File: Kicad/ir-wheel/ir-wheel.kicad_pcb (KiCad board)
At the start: 2 copper layers, 58 x 25 mm, 20 parts, among them IC1 TTE-OPB606, IC2 TTE-OPB606, K1 RIGHT, K2 LEFT, P1 BOURNS-TC33X-200K, U1 MICROCHIP-MCP6541-SOT-23

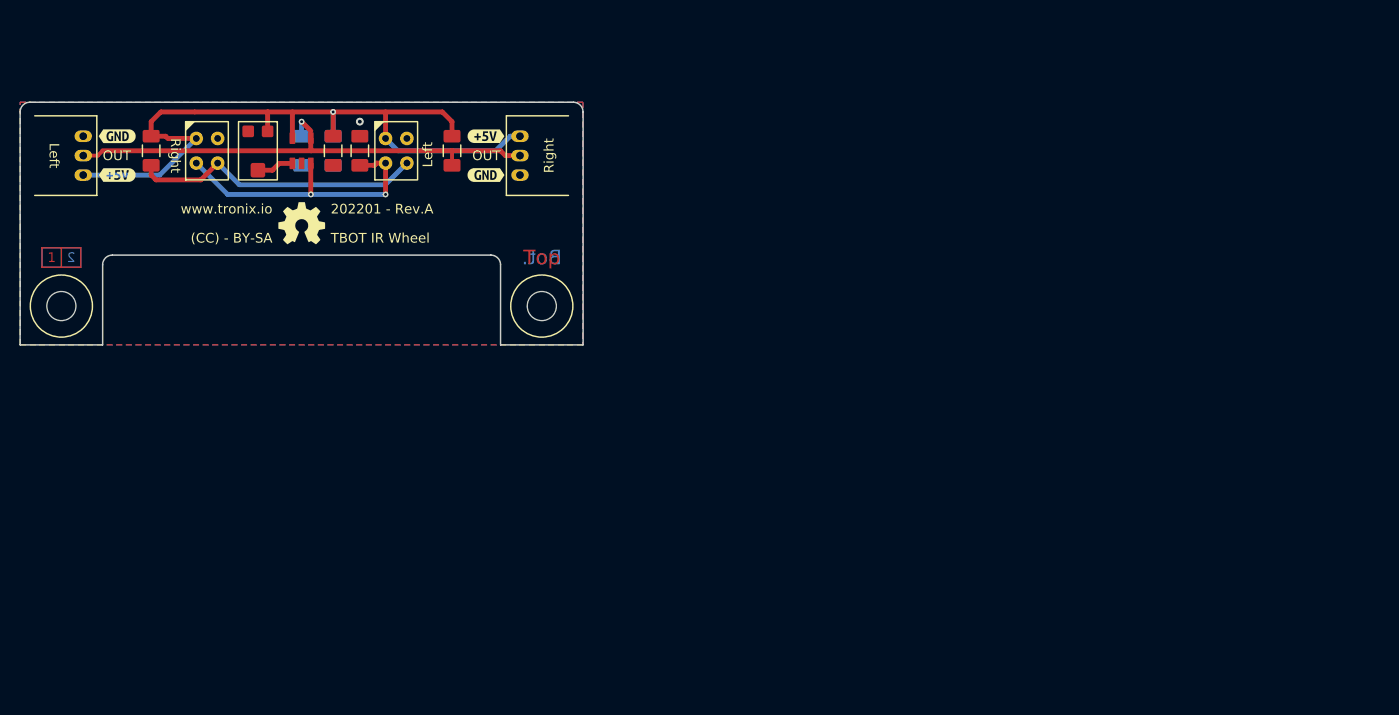
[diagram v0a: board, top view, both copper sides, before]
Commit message: Up
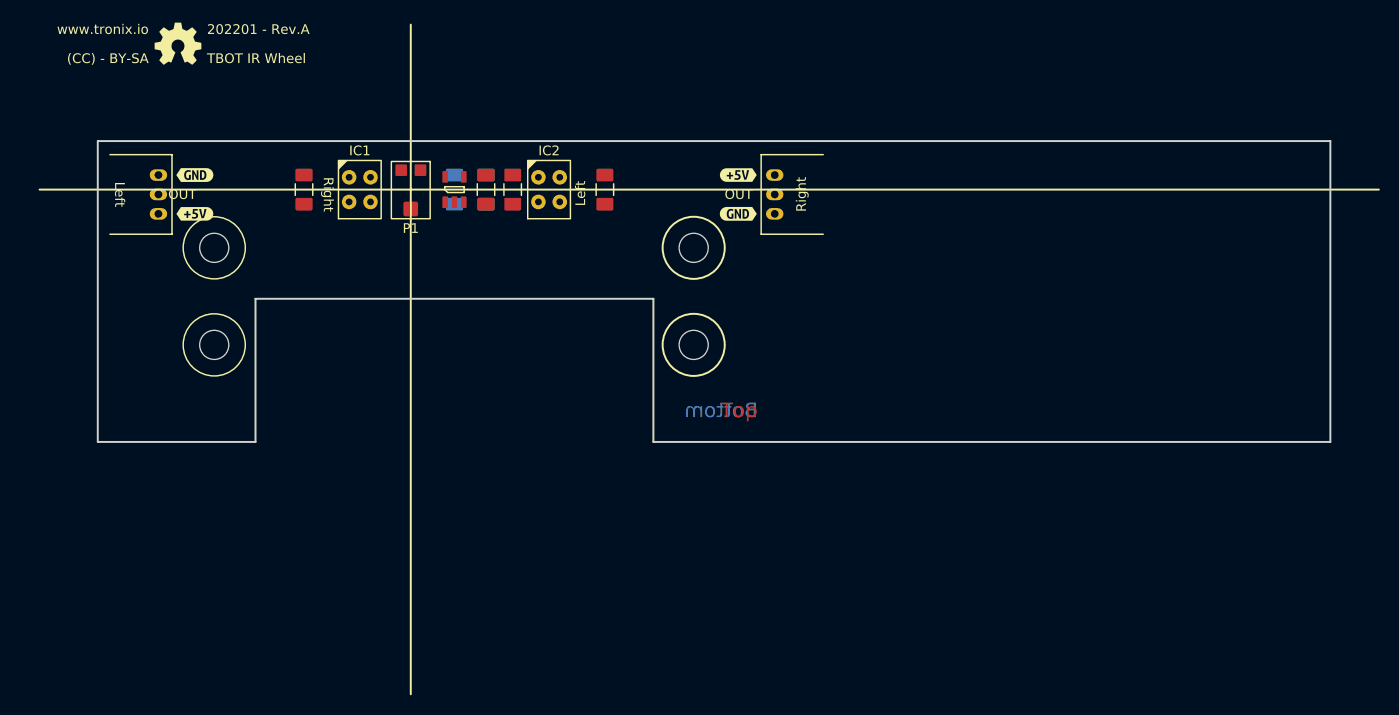
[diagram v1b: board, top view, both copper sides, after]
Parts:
- added H3: MOUNTING-HOLE-3MM-MASK, tronixio:MOUNTING-HOLE-3MM-MASK, F.Cu at (169.4, 100.0)
- added H4: MOUNTING-HOLE-3MM-MASK, tronixio:MOUNTING-HOLE-3MM-MASK, F.Cu at (169.4, 90.0)
- C1, C2, C3: footprint tronixio:CAPACITOR-1206 -> tronixio:CAPACITOR-SMD-1206
- H1, H2: value MOUNTING-HOLE-MASK-3MM -> MOUNTING-HOLE-3MM-MASK; footprint tronixio:M3-MASK -> tronixio:MOUNTING-HOLE-3MM-MASK
- IC1, IC2: value TTE-OPB606 -> OPB606; footprint tronixio:zzOPB-606 -> tronixio:OPB-606
- K1: value RIGHT -> Right
- K2: value LEFT -> Left
- P1: value BOURNS-TC33X-200K -> 200k; footprint tronixio:zzzTC33X -> tronixio:TC33X
- R1: footprint tronixio:RESISTOR-1206 -> tronixio:RESISTOR-SMD-1206
- R2: value 100K -> 100k; footprint tronixio:RESISTOR-1206 -> tronixio:RESISTOR-SMD-1206
- R3: value 10K -> 10k; footprint tronixio:RESISTOR-1206 -> tronixio:RESISTOR-SMD-1206
- U1: value MICROCHIP-MCP6541-SOT-23 -> MCP6541
- moved H2 34.0 mm to (120.0, 100.0)
- moved K2 26.6 mm to (177.8, 82.5)
- moved kibuzzard-629B8965 26.3 mm to (174.0, 82.5)
- moved kibuzzard-629B896F 26.3 mm to (174.0, 86.5)
- moved GB 22.5 mm to (116.2, 69.0)
- moved GT 22.5 mm to (116.2, 69.0)
- moved H1 16.9 mm to (120.0, 90.0)
- moved C1 16.2 mm to (148.0, 84.0)
- moved C2 16.2 mm to (148.0, 84.0)
- moved C3 16.2 mm to (144.8, 84.0)
- moved IC1 16.2 mm to (135.0, 84.0)
- moved IC2 16.2 mm to (154.5, 84.0)
- moved P1 16.2 mm to (140.2, 84.0)
- moved R1 16.2 mm to (129.2, 84.0)
- moved R2 16.2 mm to (150.8, 84.0)
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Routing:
- net +5V: track 80.2 -> 0.00 mm, vias 1 -> 0
- net Net-(C3-Pad1): track 51.1 -> 0.00 mm, vias 1 -> 0
- net Net-(IC1-ANODE): track 30.1 -> 0.00 mm
- net Net-(IC1-EMITTER): track 30.0 -> 0.00 mm, vias 2 -> 0
- net Net-(U1A-+): track 3.84 -> 0.00 mm
- net GND: vias 1 -> 0
- removed copper zone on B.Cu, net GND
- removed copper zone on F.Cu, net GND
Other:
- board size 58 x 25 mm -> 127 x 31 mm
- board text added: "Bottom"
- board text removed: "1"
- board text removed: "2"
- board text removed: "Bot."
